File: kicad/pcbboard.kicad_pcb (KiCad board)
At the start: 2 copper layers, 147 x 113.5 mm, 32 parts

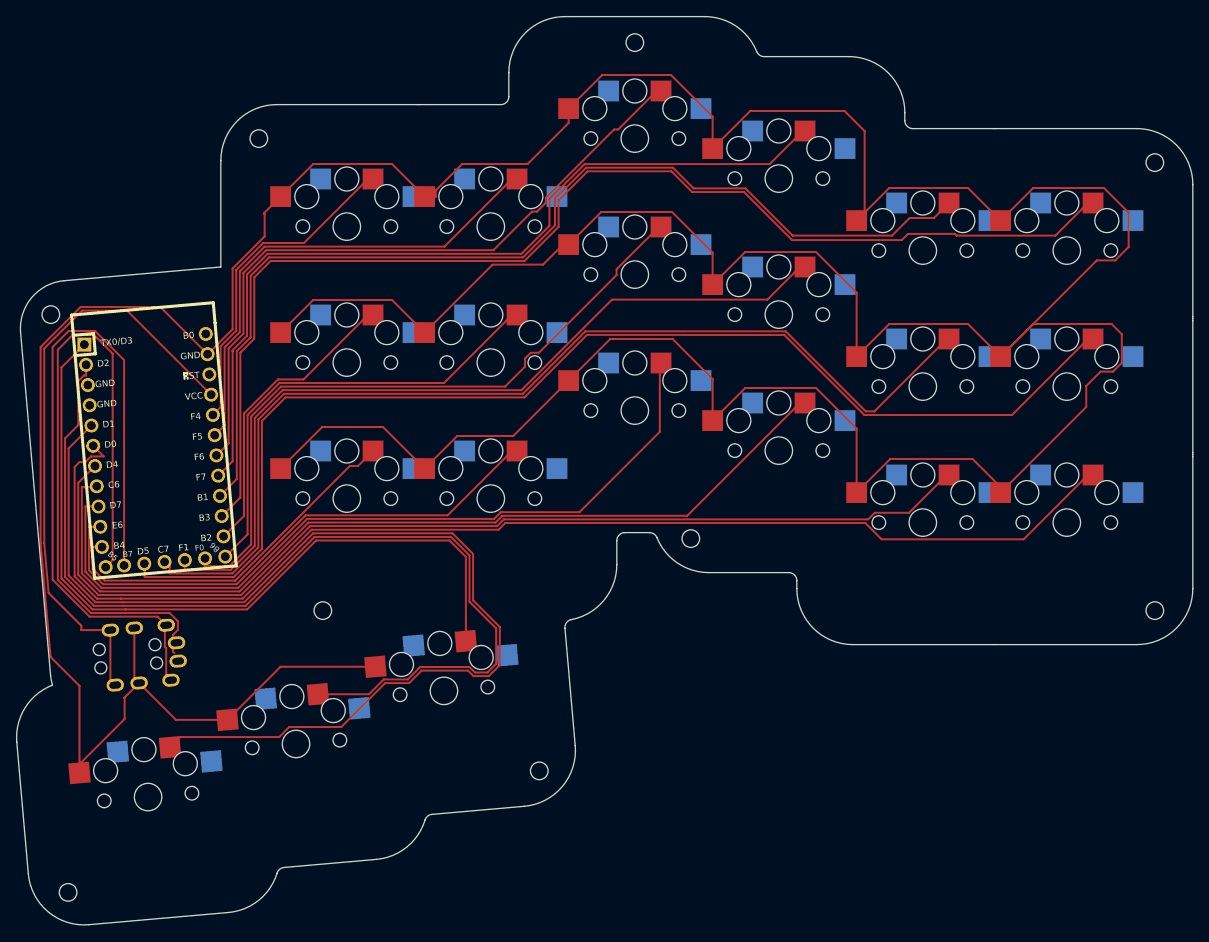
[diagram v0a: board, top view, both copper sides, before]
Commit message: Final changes pre-print
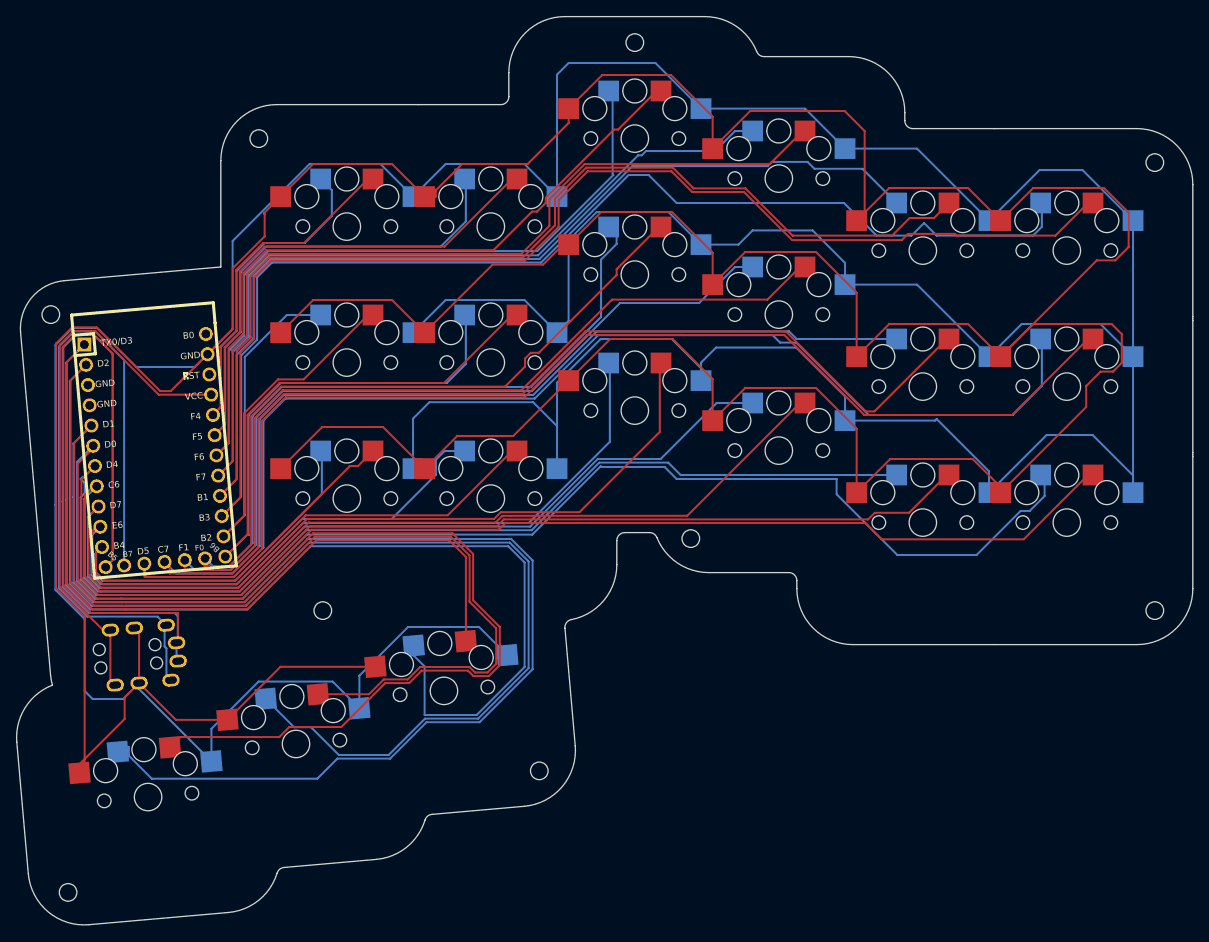
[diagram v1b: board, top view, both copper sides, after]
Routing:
- net GND: track 619.9 -> 1222.8 mm
- net thumb_left: track 137.8 -> 294.2 mm
- net matrix_outer_bottom: track 156.3 -> 311.5 mm
- net matrix_outer_center: track 150.2 -> 297.3 mm
- net thumb_middle: track 123.7 -> 267.5 mm
- net matrix_outer_top: track 149.5 -> 292.5 mm
- net thumb_right: track 97.5 -> 227.9 mm
- net matrix_pinky_bottom: track 130.6 -> 256.4 mm
- net matrix_pinky_top: track 129.1 -> 246.8 mm
- net matrix_pinky_center: track 128.9 -> 243.3 mm
- net matrix_ring_bottom: track 113.8 -> 218.8 mm
- net matrix_ring_top: track 105.8 -> 202.9 mm
- net matrix_ring_center: track 103.8 -> 200.2 mm
- net matrix_middle_bottom: track 99.2 -> 190.5 mm
- net matrix_middle_top: track 86.2 -> 172.2 mm
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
